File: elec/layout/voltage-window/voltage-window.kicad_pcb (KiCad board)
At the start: 2 copper layers, 9 parts

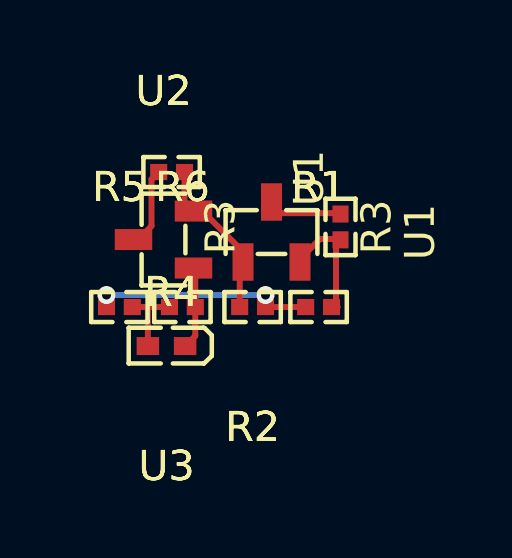
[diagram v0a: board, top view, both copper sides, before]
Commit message: fixed
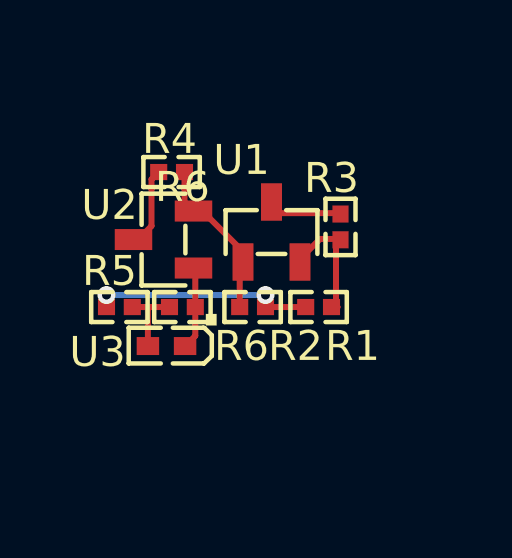
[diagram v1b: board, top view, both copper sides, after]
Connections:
- net REF-1 renamed K
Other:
- board text added: "."
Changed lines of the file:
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@@
 	(net 1 "gnd")
 	(net 2 "A")
-	(net 3 "REF-1")
+	(net 3 "K")
 	(net 4 "REF")
 	(net 5 "hv")
@@
 		(at 44.8 29.3 180)
 		(property "Reference" "U3"
-			(at 0 -4 0)
+			(at 2.3 -0.2 0)
 			(layer "F.SilkS")
 			(effects
@@
 			(fill no)
 			(layer "F.Fab")
-		)
-		(fp_text user "${REFERENCE}"
-			(at 0 -4 0)
-			(layer "F.SilkS")
-			(effects
-				(font
-					(size 1 1)
-					(thickness 0.15)
-				)
-			)
 		)
 		(fp_text user "${REFERENCE}"
@@
 		(at 44.97 23.5 180)
 		(property "Reference" "R4"
-			(at 0 -4 0)
+			(at 0.07 1.1 0)
 			(layer "F.SilkS")
 			(effects
@@
 			(fill no)
 			(layer "F.Fab")
-		)
-		(fp_text user "${REFERENCE}"
-			(at 0 -4 0)
-			(layer "F.SilkS")
-			(effects
-				(font
-					(size 1 1)
-					(thickness 0.15)
-				)
-			)
 		)
 		(fp_text user "${REFERENCE}"
@@
 			(size 0.57 0.54)
 			(layers "F.Cu" "F.Mask" "F.Paste")
-			(net 3 "REF-1")
+			(net 3 "K")
 		)
 		(pad "2" smd rect
@@
 		(at 47.67 28 180)
 		(property "Reference" "R2"
-			(at 0 -4 0)
+			(at -1.43 -1.3 0)
 			(layer "F.SilkS")
 			(effects
@@
 			(fill no)
 			(layer "F.Fab")
-		)
-		(fp_text user "${REFERENCE}"
-			(at 0 -4 0)
-			(layer "F.SilkS")
-			(effects
-				(font
-					(size 1 1)
-					(thickness 0.15)
-				)
-			)
 		)
 		(fp_text user "${REFERENCE}"
@@
 			(size 0.57 0.54)
 			(layers "F.Cu" "F.Mask" "F.Paste")
-			(net 3 "REF-1")
+			(net 3 "K")
 		)
 		(embedded_fonts no)
@@
 		(at 45.33 28)
 		(property "Reference" "R6"
-			(at 0 -4 0)
+			(at 1.97 1.3 0)
 			(layer "F.SilkS")
 			(effects
@@
 		(at 48.3 25.5 -90)
 		(property "Reference" "U1"
-			(at -1.8 -1.25 90)
+			(at -2.4 1 180)
 			(layer "F.SilkS")
 			(effects
@@
 			(fill no)
 			(layer "F.Fab")
-		)
-		(fp_text user "${REFERENCE}"
-			(at 0 -4.95 90)
-			(layer "F.SilkS")
-			(effects
-				(font
-					(size 1 1)
-					(thickness 0.15)
-				)
-			)
 		)
 		(fp_text user "${REFERENCE}"
@@
 			(size 1.25 0.7)
 			(layers "F.Cu" "F.Mask" "F.Paste")
-			(net 3 "REF-1")
+			(net 3 "K")
 		)
 		(pad "2" smd rect
@@
 		(at 49.87 28)
 		(property "Reference" "R1"
-			(at 0 -4 0)
+			(at 1.13 1.3 0)
 			(layer "F.SilkS")
 			(effects
@@
 			(fill no)
 			(layer "F.Fab")
-		)
-		(fp_text user "${REFERENCE}"
-			(at 0 -4 0)
-			(layer "F.SilkS")
-			(effects
-				(font
-					(size 1 1)
-					(thickness 0.15)
-				)
-			)
 		)
 		(fp_text user "${REFERENCE}"
@@
 		(at 43.23 28)
 		(property "Reference" "R5"
-			(at 0 -4 0)
+			(at -0.33 -1.2 0)
 			(layer "F.SilkS")
 			(effects
@@
 			(fill no)
 			(layer "F.Fab")
-		)
-		(fp_text user "${REFERENCE}"
-			(at 0 -4 0)
-			(layer "F.SilkS")
-			(effects
-				(font
-					(size 1 1)
-					(thickness 0.15)
-				)
-			)
 		)
 		(fp_text user "${REFERENCE}"
@@
 		(at 44.7 25.75)
 		(property "Reference" "U2"
-			(at 0 -4.95 0)
+			(at -1.8 -1.15 0)
 			(layer "F.SilkS")
 			(effects
@@
 			(fill no)
 			(layer "F.Fab")
-		)
-		(fp_text user "${REFERENCE}"
-			(at 0 -4.95 0)
-			(layer "F.SilkS")
-			(effects
-				(font
-					(size 1 1)
-					(thickness 0.15)
-				)
-			)
 		)
 		(fp_text user "${REFERENCE}"
@@
 			(size 1.25 0.7)
 			(layers "F.Cu" "F.Mask" "F.Paste")
-			(net 3 "REF-1")
+			(net 3 "K")
 		)
 		(pad "3" smd rect
@@
 			(at 0 -4 90)
 			(layer "F.SilkS")
+			(hide yes)
 			(effects
 				(font
@@
 		)
 		(fp_text user "${REFERENCE}"
-			(at 0 1.2 90)
+			(at 1.63 -0.3 180)
 			(layer "F.SilkS")
 			(effects
@@
 		(embedded_fonts no)
 	)
+	(gr_text "."
+		(at 45.9 28.8 0)
+		(layer "F.SilkS")
+		(effects
+			(font
+				(size 1.5 1.5)
+				(thickness 0.3)
+				(bold yes)
+			)
+			(justify left bottom)
+		)
+	)
 	(segment
